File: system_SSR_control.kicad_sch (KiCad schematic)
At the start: 12 parts, among them Q1 2.1V, Q2 2N7000, Q3 2N7000, SW1 FSM2JSMA, SW2 FSM2JSMA

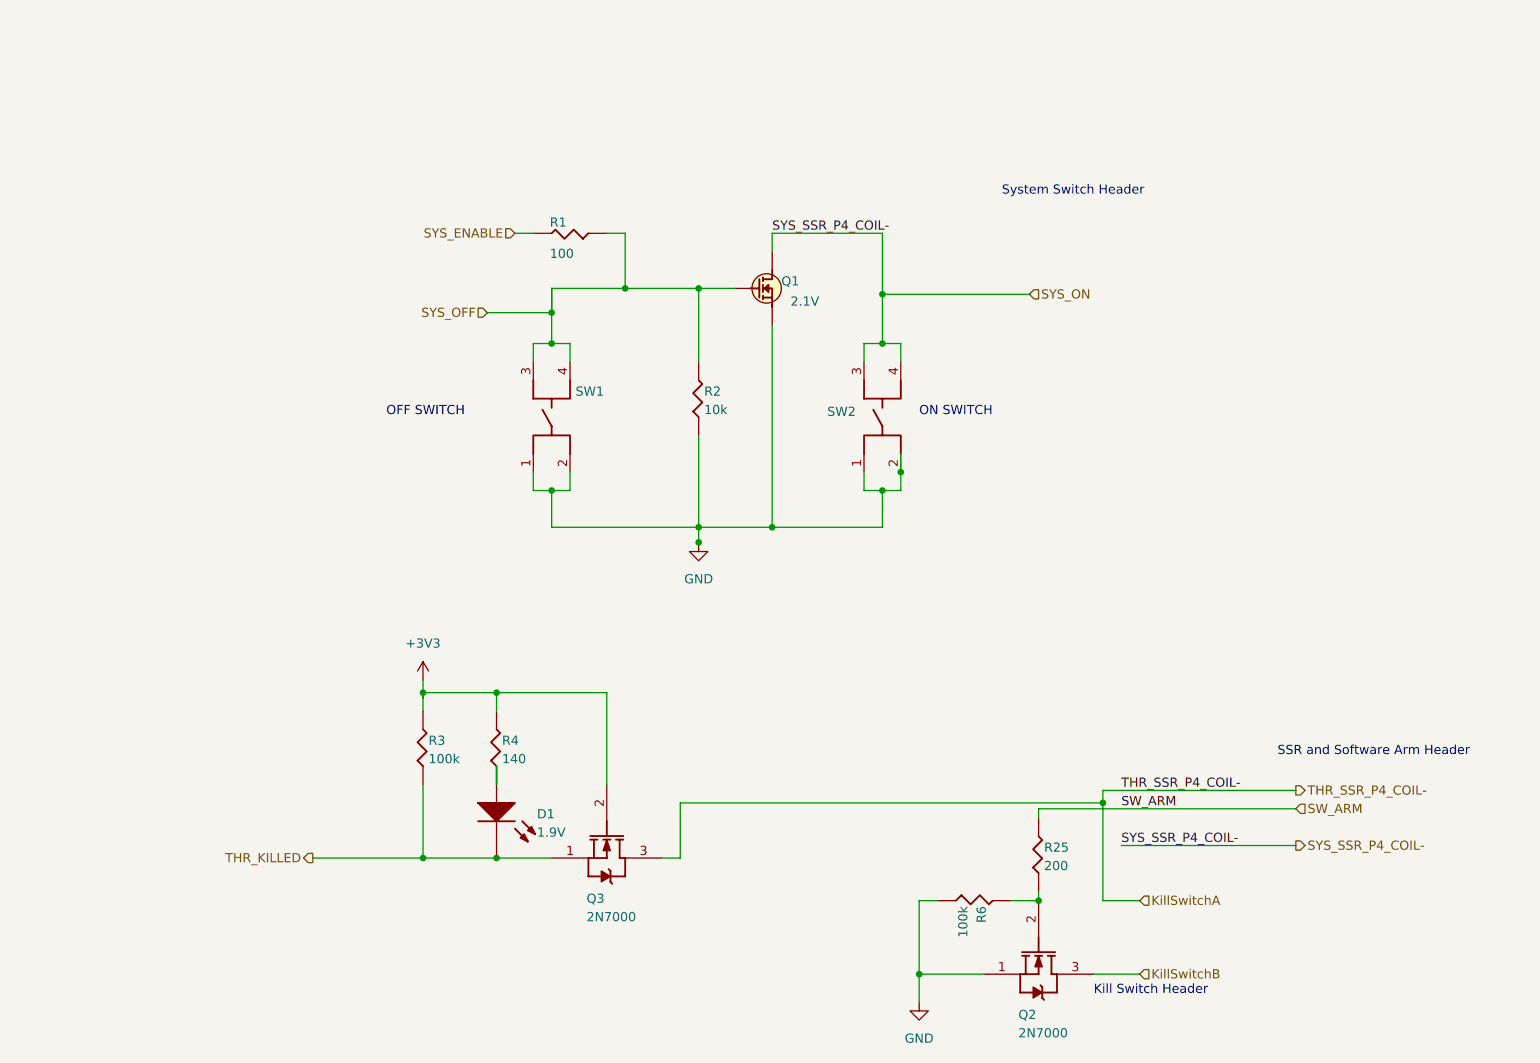
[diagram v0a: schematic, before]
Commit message: Fix a variety of small issues
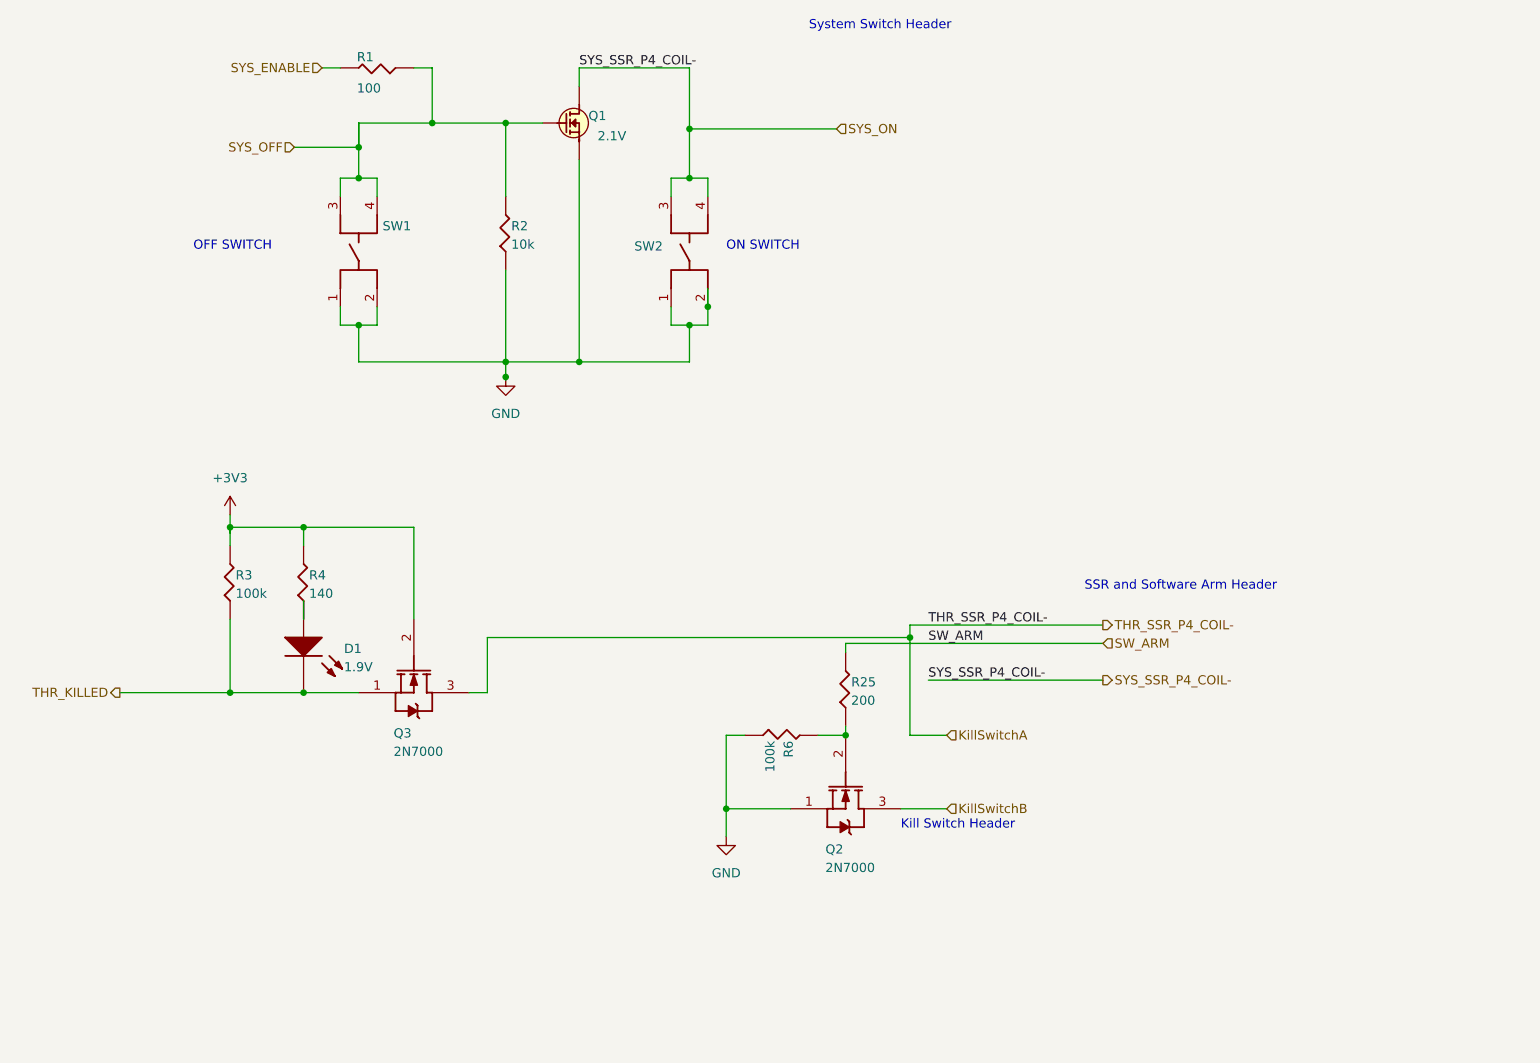
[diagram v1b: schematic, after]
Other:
- moved on the sheet: D1, Q1, Q2, Q3, R1, R2, R25, R3, R4, R6, SW1, SW2
